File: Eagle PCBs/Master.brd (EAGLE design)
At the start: 100 x 80 mm, 12 parts

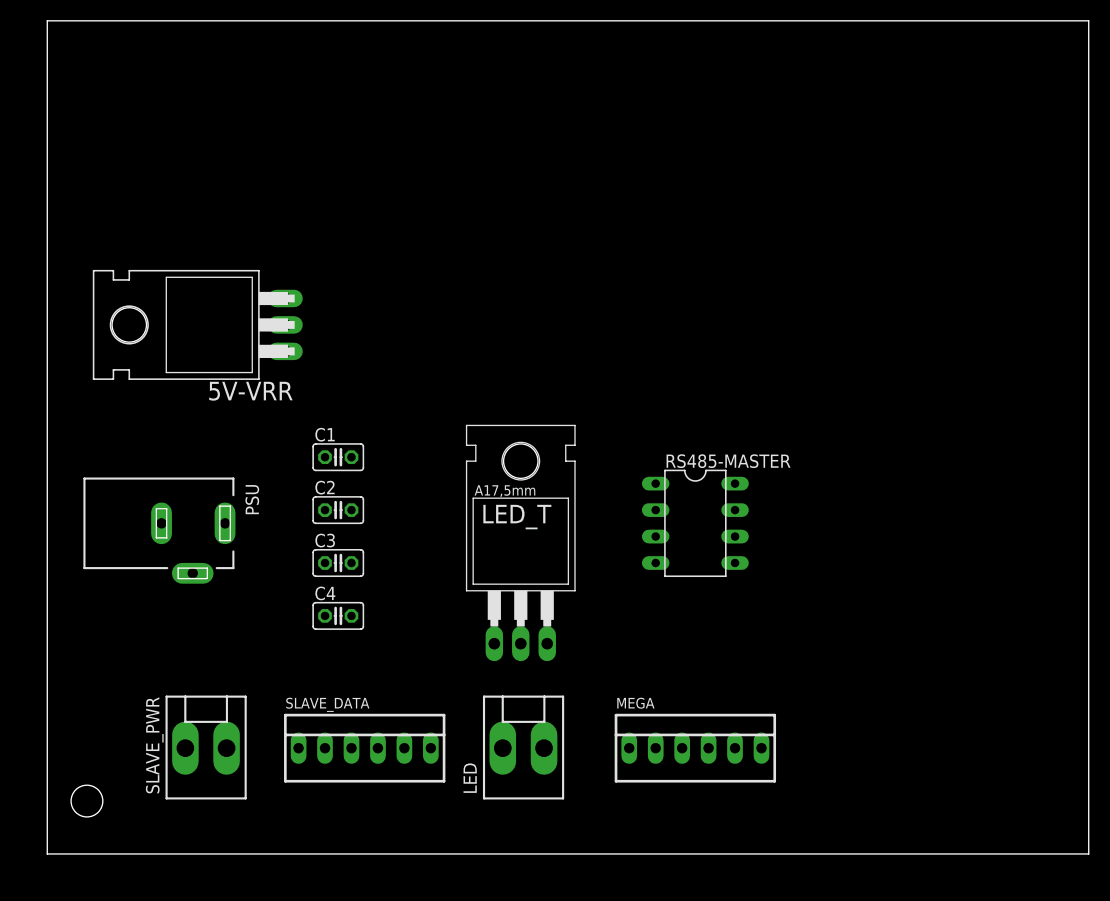
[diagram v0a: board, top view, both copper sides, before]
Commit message: Master PCB WIP
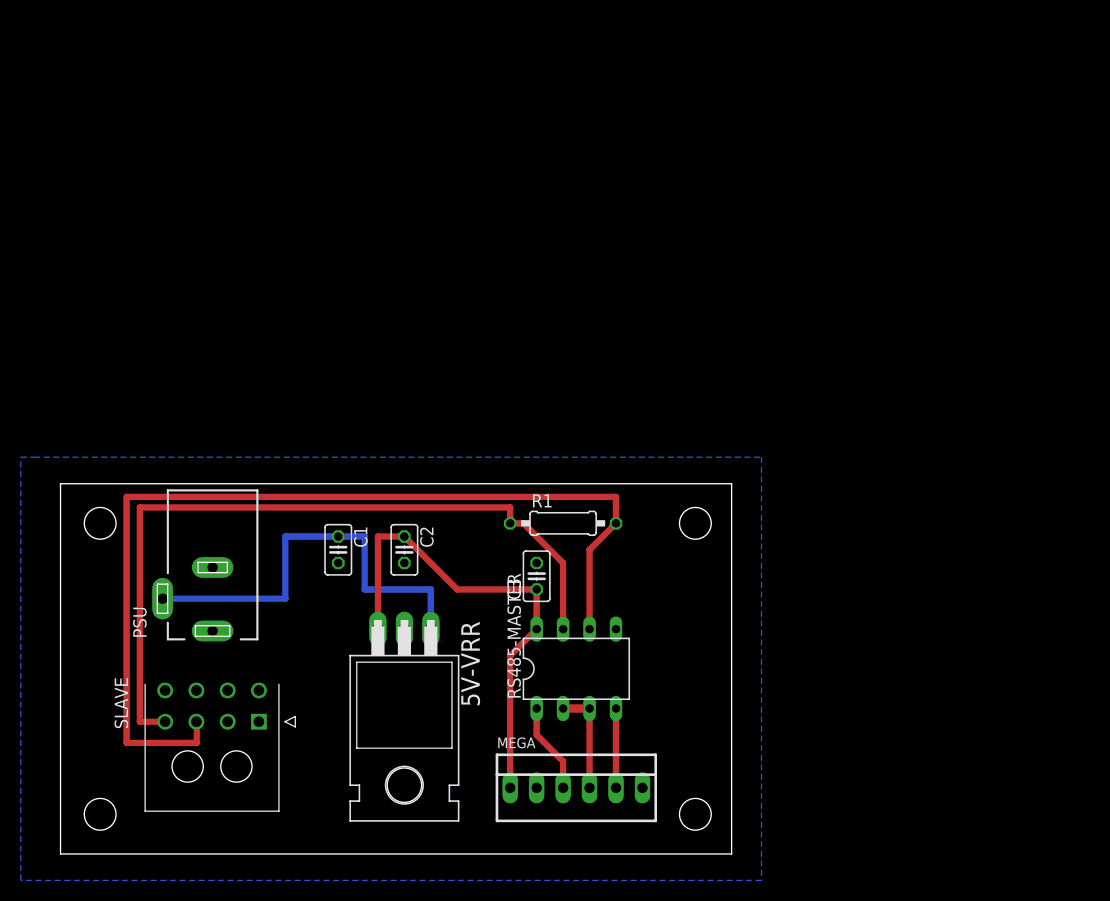
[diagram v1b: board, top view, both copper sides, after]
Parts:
- removed C4: 22uF 16V, rcl:C025-025X050
- removed LED, SLAVE_PWR: (no value), con-molex:KK-156-2
- removed LED_T: BD239, transistor-neu-to92:TO220
- removed SLAVE_DATA: (no value), con-molex:22-23-2061
- added R1: 120Ω, rcl:0207/10
- added SLAVE: 212528-0801, SamacSys_Parts:212528-08YY
- 5V-VRR: value 7805T -> L7805CV
- C1: value 220uF 16V -> 0.33uF
- moved 5V-VRR 44.9 mm to (34.3, 11.4), turned to 180 degrees
- moved C3 19.1 mm to (47.0, 26.7), turned to 90 degrees
- moved RS485-MASTER 18.1 mm to (50.8, 17.8), turned to 0 degrees
- moved MEGA 12.0 mm to (50.8, 6.35)
- moved C1 8.89 mm to (27.9, 29.2), turned to 270 degrees
- moved PSU 7.49 mm to (15.9, 24.5), turned to 180 degrees
- moved C2 7.41 mm to (34.3, 29.2), turned to 270 degrees
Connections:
- removed net 12VCC: 5V-VRR.1, C1.1, C2.1, LED.1, PSU.2, SLAVE_PWR.1
- removed net LED_DIM: LED_T.1
- removed net LED_GND: LED.2, LED_T.2
- new net VDD: 5V-VRR.3, C2.1, C3.1, MEGA.1, RS485-MASTER.8
- net GND: now also SLAVE.7; no longer C4.2, LED_T.3, SLAVE_PWR.2
- net MEGA_P18: now also MEGA.5; no longer MEGA.4
- net MEGA_P19: now also MEGA.3; no longer MEGA.5
- net MEGA_P2: now also MEGA.4; no longer MEGA.3
- net RS485_A: now also R1.2, SLAVE.3; no longer SLAVE_DATA.1
- net RS485_B: now also R1.1, SLAVE.4; no longer SLAVE_DATA.2
- net VCC: now also 5V-VRR.1, C1.1, PSU.2, SLAVE.8; no longer 5V-VRR.3, C3.1, C4.1, MEGA.1, RS485-MASTER.8
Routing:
- net RS485_A: track 0.00 -> 93.1 mm
- net RS485_B: track 0.00 -> 73.1 mm
- net VDD: track 0.00 -> 46.3 mm
- net VCC: track 0.00 -> 40.6 mm
- net MEGA_P2: track 0.00 -> 10.2 mm
- net MEGA_P19: track 0.00 -> 8.67 mm
- net MEGA_P18: track 0.00 -> 7.62 mm
- added copper zone on layer 16, net GND
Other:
- board size 100 x 80 mm -> 64.4 x 35.5 mm
